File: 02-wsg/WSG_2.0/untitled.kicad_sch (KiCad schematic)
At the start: 33 parts, among them IC1 W25N04KVZEIR, IC3 MIC5504-3.3YM5-TR, IC8 SPX3819S-L_TR, J1 USB4110-GF-A, J4 Conn_01x02, U1 BQ21040DBVR

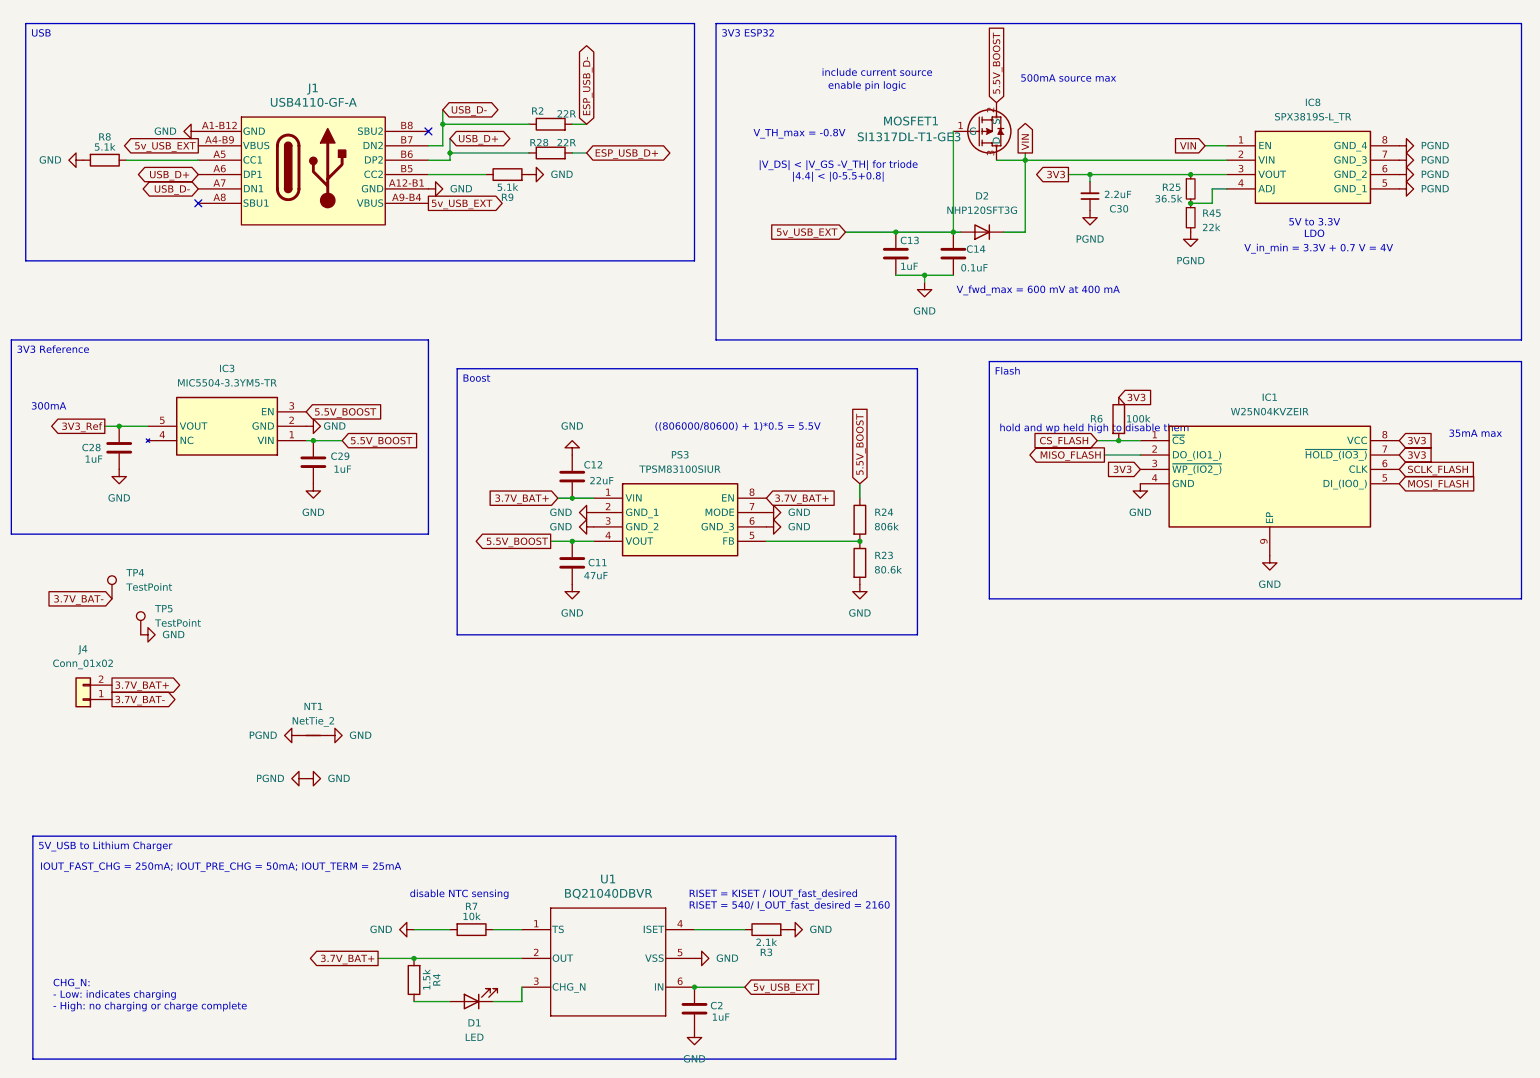
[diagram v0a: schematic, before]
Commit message: Edited comments/flag titles
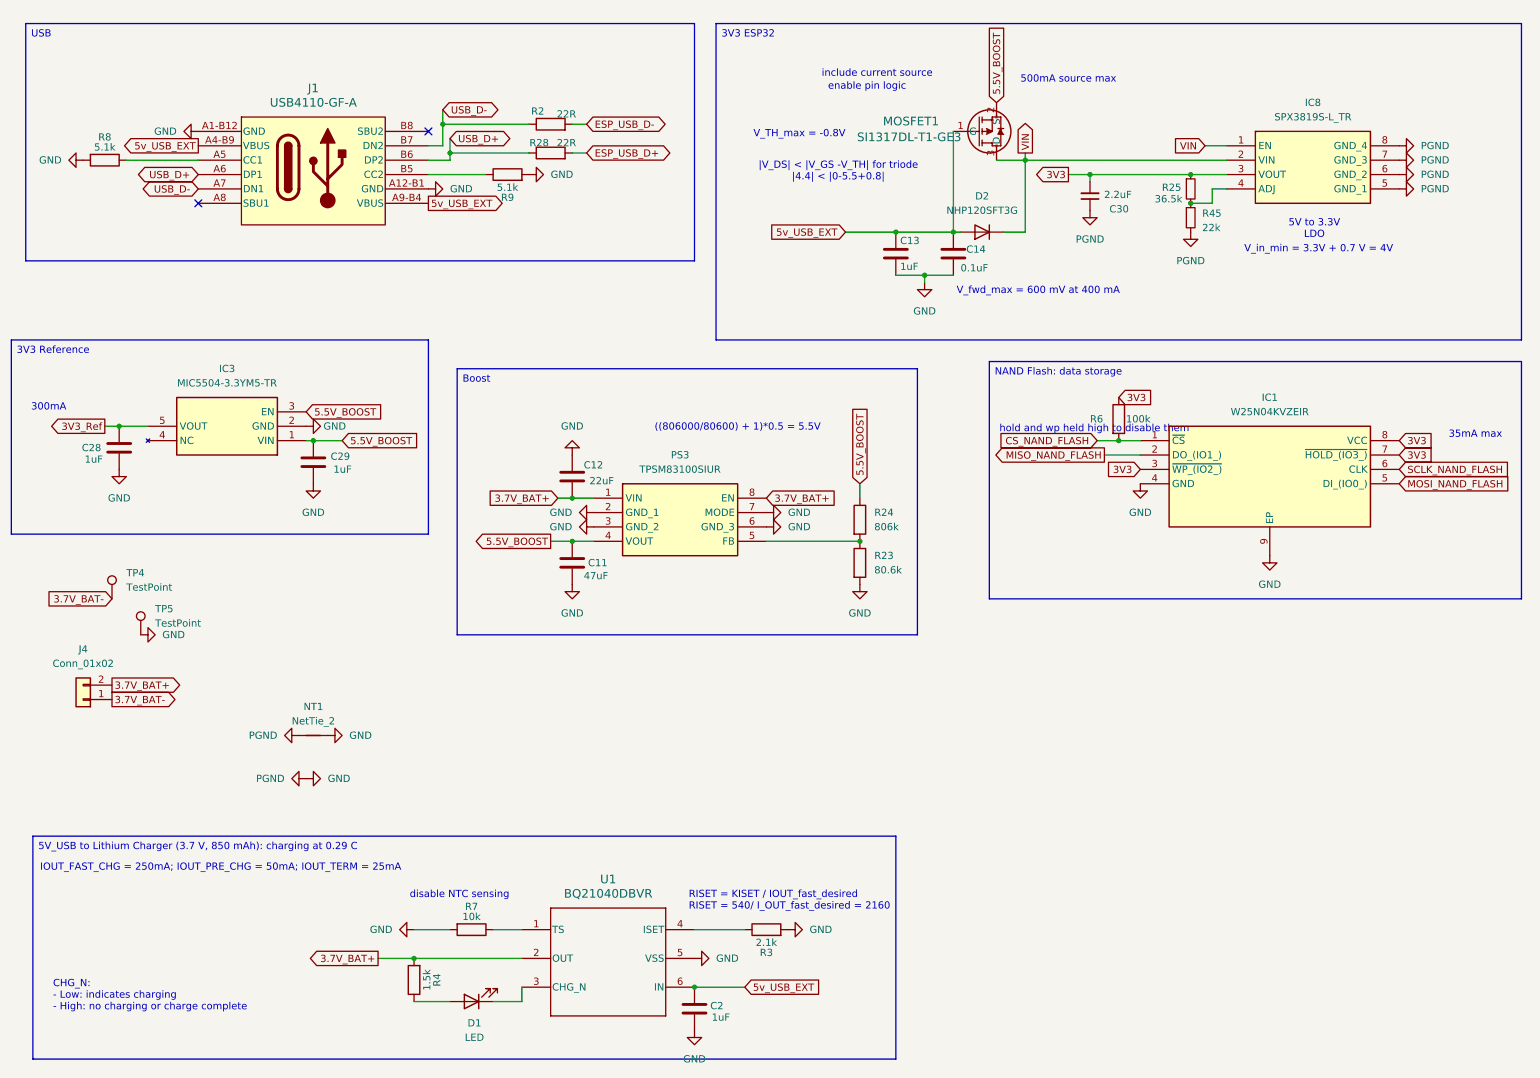
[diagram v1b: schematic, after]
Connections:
- net CS_FLASH renamed CS_NAND_FLASH
- net MISO_FLASH renamed MISO_NAND_FLASH
- net MOSI_FLASH renamed MOSI_NAND_FLASH
- net SCLK_FLASH renamed SCLK_NAND_FLASH
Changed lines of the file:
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@@
 		)
 	)
-	(text_box "Flash"
+	(text_box "NAND Flash: data storage"
 		(exclude_from_sim no)
 		(at 186.69 72.39 0)
@@
 		)
 	)
-	(text_box "5V_USB to Lithium Charger"
+	(text_box "5V_USB to Lithium Charger (3.7 V, 850 mAh): charging at 0.29 C"
 		(exclude_from_sim no)
 		(at 17.78 156.21 0)
@@
 		)
 	)
-	(global_label "CS_FLASH"
+	(global_label "CS_NAND_FLASH"
 		(shape input)
 		(at 205.74 86.36 180)
@@
 		)
 		(property "Intersheetrefs" "${INTERSHEET_REFS}"
-			(at 193.5624 86.36 0)
+			(at 187.5752 86.36 0)
 			(effects
 				(font
@@
 	(global_label "ESP_USB_D-"
 		(shape bidirectional)
-		(at 115.57 30.48 90)
-		(fields_autoplaced yes)
-		(effects
-			(font
-				(size 1.27 1.27)
-			)
-			(justify left)
-		)
-		(property "Intersheetrefs" "${INTERSHEET_REFS}"
-			(at 115.57 14.1674 90)
+		(at 115.57 30.48 0)
+		(fields_autoplaced yes)
+		(effects
+			(font
+				(size 1.27 1.27)
+			)
+			(justify left)
+		)
+		(property "Intersheetrefs" "${INTERSHEET_REFS}"
+			(at 131.8826 30.48 0)
 			(effects
 				(font
@@
 		)
 	)
-	(global_label "SCLK_FLASH"
+	(global_label "SCLK_NAND_FLASH"
 		(shape input)
 		(at 259.08 91.44 0)
@@
 		)
 		(property "Intersheetrefs" "${INTERSHEET_REFS}"
-			(at 273.5557 91.44 0)
+			(at 279.5429 91.44 0)
 			(effects
 				(font
@@
 		)
 	)
-	(global_label "MISO_FLASH"
+	(global_label "MISO_NAND_FLASH"
 		(shape output)
 		(at 207.01 88.9 180)
@@
 		)
 		(property "Intersheetrefs" "${INTERSHEET_REFS}"
-			(at 192.7157 88.9 0)
+			(at 186.7285 88.9 0)
 			(effects
 				(font
@@
 		)
 	)
-	(global_label "MOSI_FLASH"
+	(global_label "MOSI_NAND_FLASH"
 		(shape input)
 		(at 259.08 93.98 0)
@@
 		)
 		(property "Intersheetrefs" "${INTERSHEET_REFS}"
-			(at 273.3743 93.98 0)
-			(effects
-				(font
+			(at 279.3615 93.98 0)
+			(effects
+				(font
